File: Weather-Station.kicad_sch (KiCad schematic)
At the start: 3 parts, among them J1 Conn_01x22, J2 Conn_01x22, U1 ESP32-S3-DevKitC

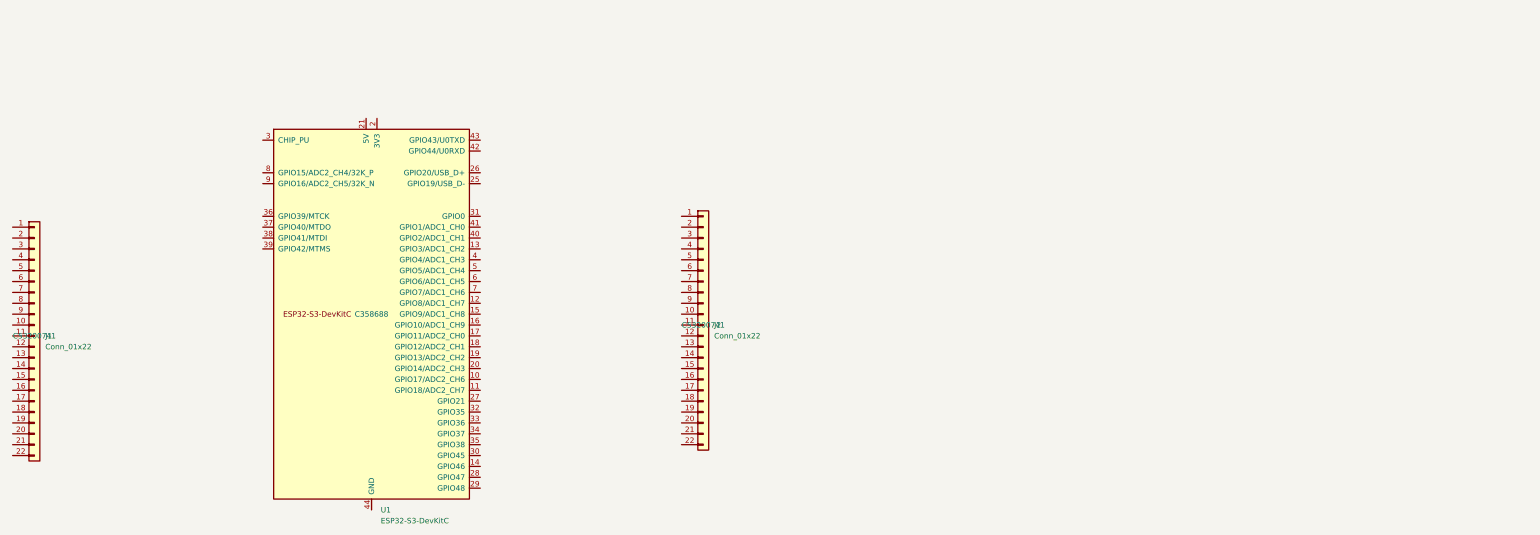
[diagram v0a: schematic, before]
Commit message: WIP: Finding pin headers/rows
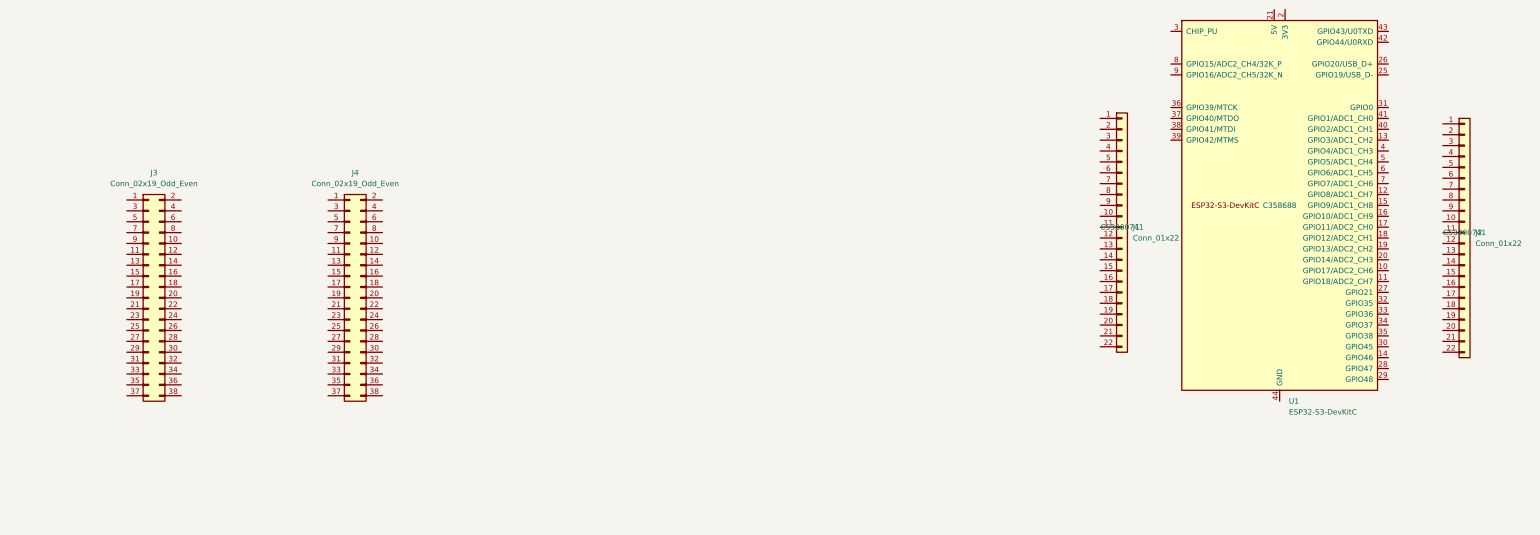
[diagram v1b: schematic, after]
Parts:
- added J3, J4: Conn_02x19_Odd_Even, Connector_PinHeader_2.54mm:PinHeader_2x19_P2.54mm_Vertical, symbol Connector_Generic:Conn_02x19_Odd_Even
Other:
- moved on the sheet: J1, J2, U1
